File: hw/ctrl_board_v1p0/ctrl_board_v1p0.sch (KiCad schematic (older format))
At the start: 33 parts, among them J1 RaSCSI Connector, J2 OLED Connector, J3 Conn_01x04_Male, P1 Conn_02x20_Odd_Even, SW1 SW_SPST, SW2 SW_SPST, SW3 SW_SPST, SW4 Rotary_Encoder_Switch, U1 PCA9554APW,118

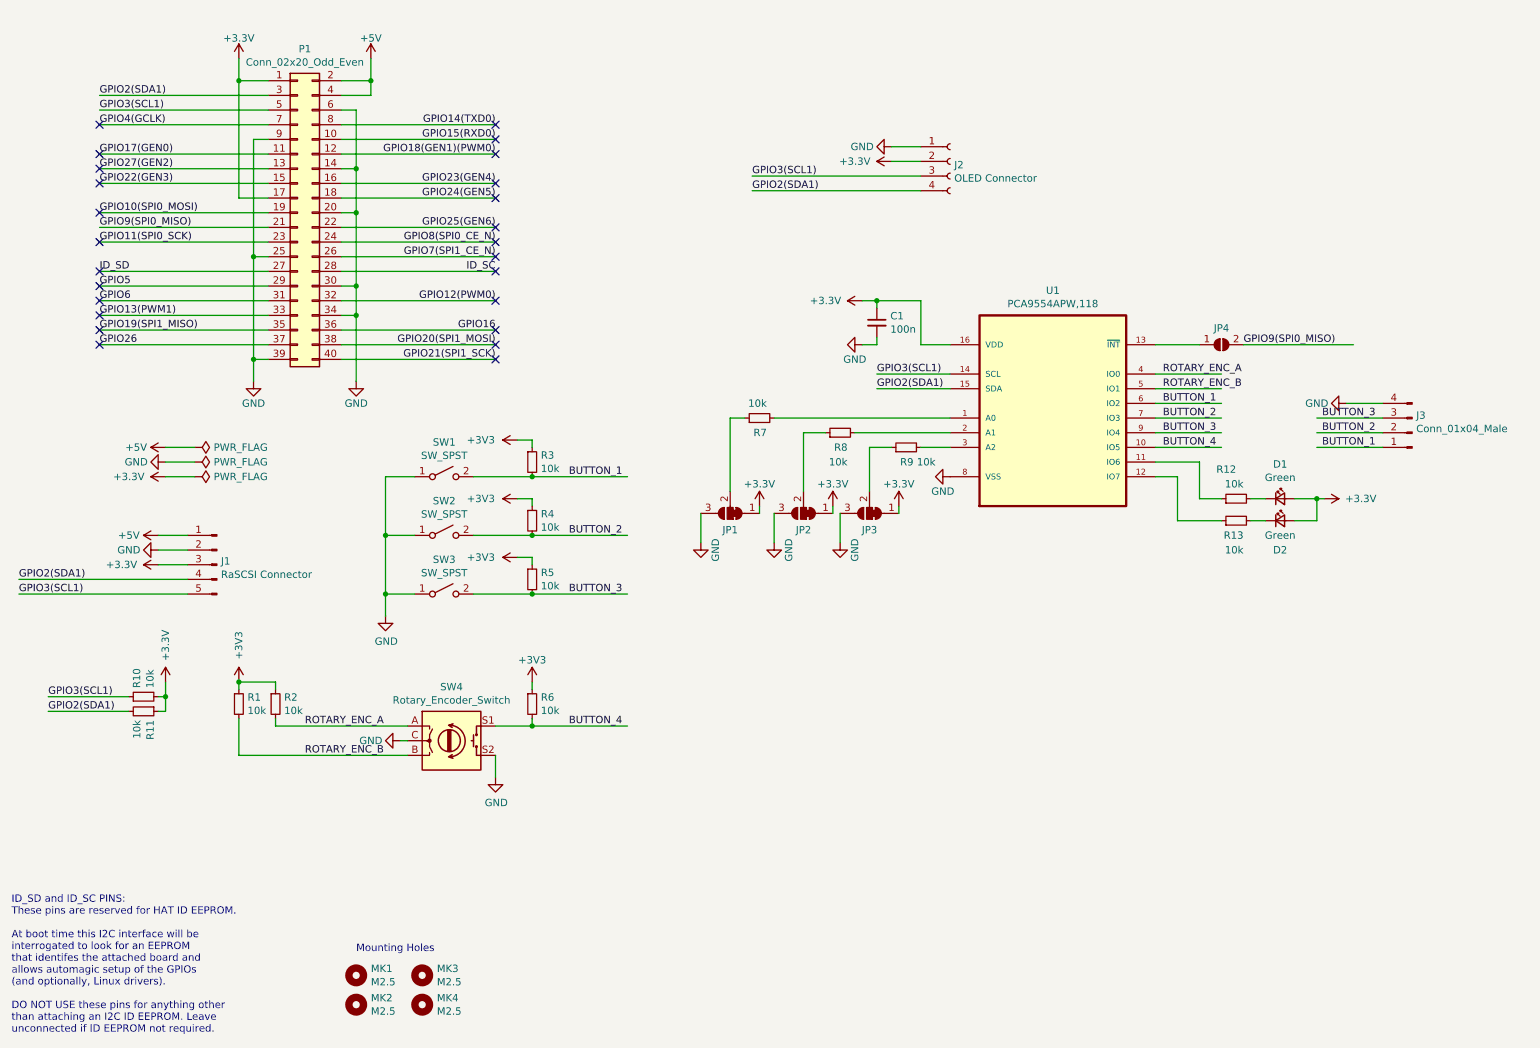
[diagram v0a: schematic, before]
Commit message: cleaned up layout
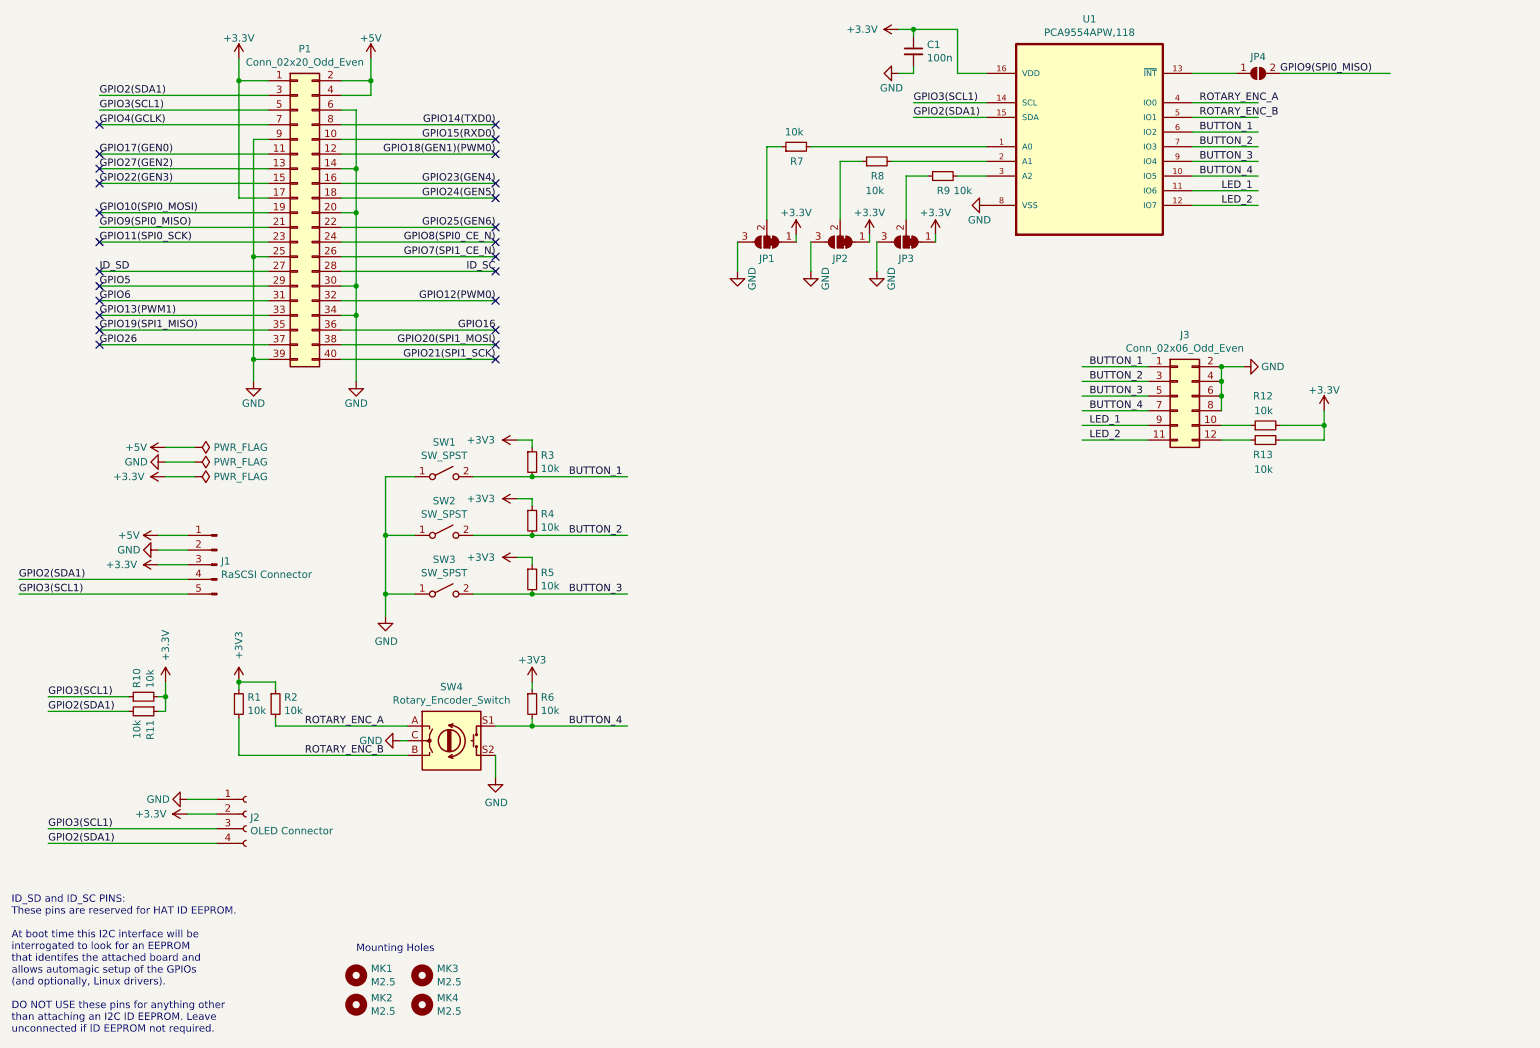
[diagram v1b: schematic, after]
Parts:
- removed D1, D2: Green, LED_SMD:LED_0805_2012Metric, symbol Device:LED_Small
- removed J3: Conn_01x04_Male, Connector_PinHeader_2.54mm:PinHeader_1x04_P2.54mm_Vertical, symbol Connector:Conn_01x04_Male
- added J3: Conn_02x06_Odd_Even, Connector_PinHeader_2.54mm:PinHeader_2x06_P2.54mm_Vertical, symbol Connector_Generic:Conn_02x06_Odd_Even
- J2: footprint Connector_PinSocket_2.54mm:PinSocket_1x04_P2.54mm_Vertical -> mousebites:OLED_Footprint
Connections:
- net labels added: LED_1, LED_2
- wire segments 149 -> 151
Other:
- moved on the sheet: C1, J2, JP1, JP2, JP3, JP4, R12, R13, R7, R8, R9, U1
